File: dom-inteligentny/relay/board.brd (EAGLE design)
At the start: 92.7 x 87.6 mm, 77 parts, among them K1 OMRON-G3MB-202P-SSR, K10 OMRON-G3MB-202P-SSR, K11 OMRON-G3MB-202P-SSR, K12 OMRON-G3MB-202P-SSR, K13 OMRON-G3MB-202P-SSR, K14 OMRON-G3MB-202P-SSR, K15 OMRON-G3MB-202P-SSR, K16 OMRON-G3MB-202P-SSR, K17 691218410003, K18 691218410003, K19 691218410003, K2 OMRON-G3MB-202P-SSR, K20 691218410003, K21 691218410003, K22 691218410003, K3 OMRON-G3MB-202P-SSR, K4 OMRON-G3MB-202P-SSR, K5 OMRON-G3MB-202P-SSR, K6 OMRON-G3MB-202P-SSR, K7 OMRON-G3MB-202P-SSR, K8 OMRON-G3MB-202P-SSR, K9 OMRON-G3MB-202P-SSR, T1 BC847, T10 BC847, T11 BC847, T12 BC847, T13 BC847, T14 BC847, T15 BC847, T16 BC847, T2 BC847, T3 BC847, T4 BC847, T5 BC847, T6 BC847, T7 BC847, T8 BC847, T9 BC847, X1 GLX-S-88M

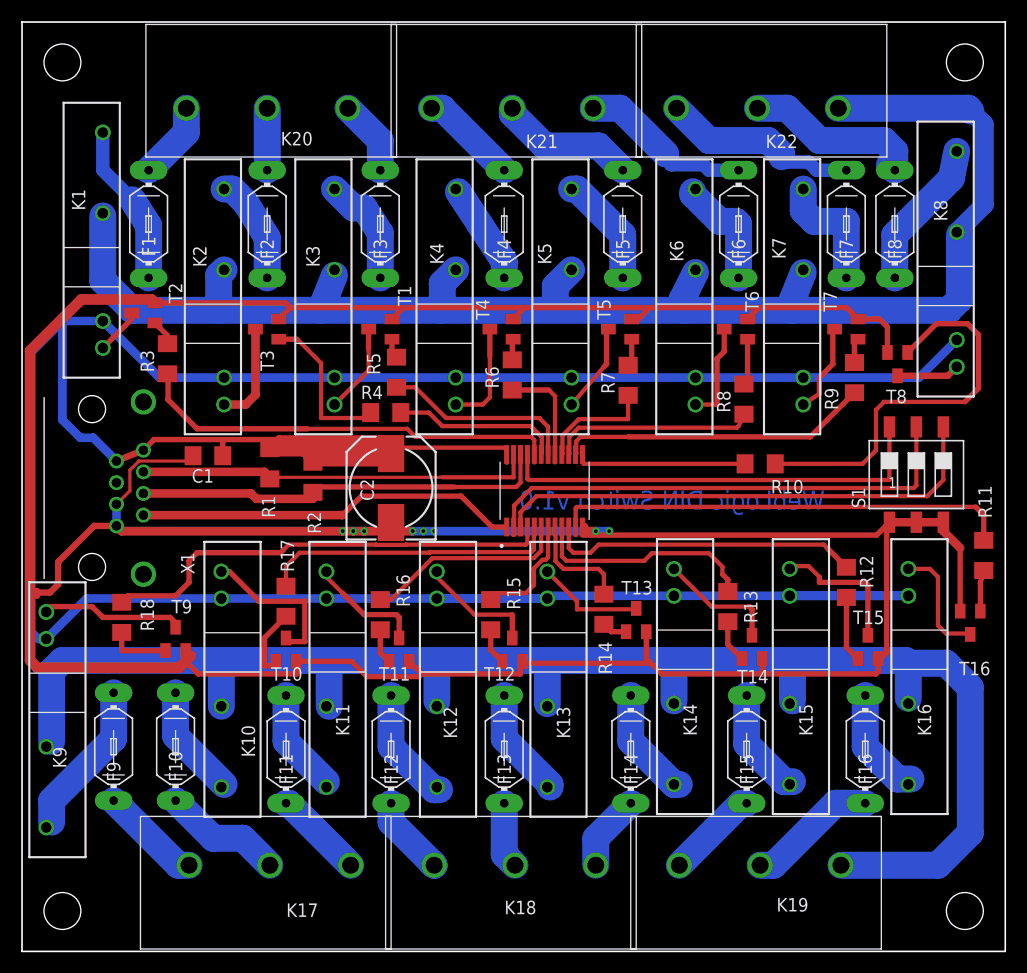
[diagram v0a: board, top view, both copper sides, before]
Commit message: new files
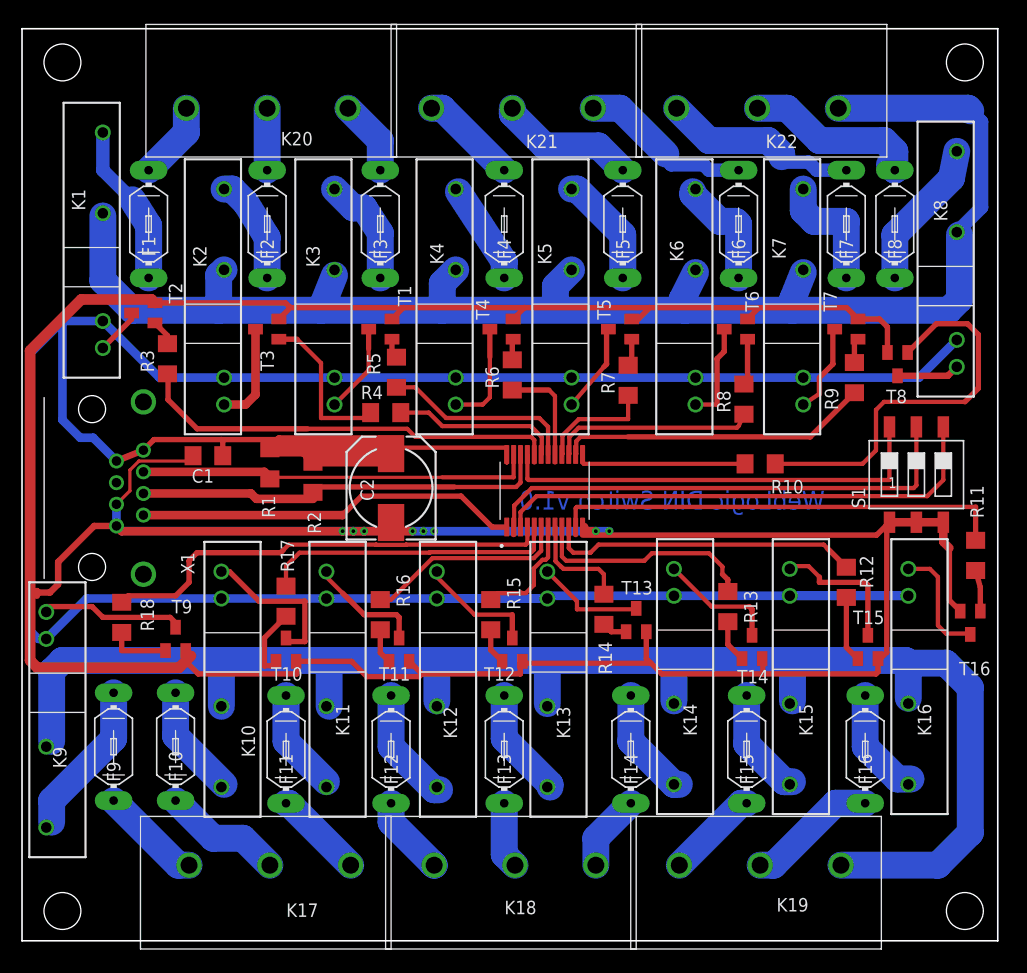
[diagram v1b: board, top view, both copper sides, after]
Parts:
- moved R11 0.76 mm to (89.9, 37.3)
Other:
- board size 92.7 x 87.6 mm -> 92 x 86 mm
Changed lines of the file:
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@@
 <setting verticaltext="up"/>
 </settings>
-<grid distance="10" unitdist="mil" unit="mil" style="lines" multiple="1" display="no" altdistance="5" altunitdist="mil" altunit="mil"/>
+<grid distance="1" unitdist="mm" unit="mm" style="lines" multiple="1" display="no" altdistance="1" altunitdist="mm" altunit="mm"/>
 <layers>
 <layer number="1" name="Top" color="4" fill="1" visible="yes" active="yes"/>
@@
 <board>
 <plain>
-<wire x1="0" y1="0" x2="0" y2="87.63" width="0.1524" layer="20"/>
-<wire x1="0" y1="87.63" x2="92.71" y2="87.63" width="0.1524" layer="20"/>
-<wire x1="92.71" y1="87.63" x2="92.71" y2="0" width="0.1524" layer="20"/>
-<wire x1="92.71" y1="0" x2="0" y2="0" width="0.1524" layer="20"/>
+<wire x1="0" y1="1" x2="0" y2="87" width="0.1524" layer="20"/>
+<wire x1="0" y1="87" x2="92" y2="87" width="0.1524" layer="20"/>
+<wire x1="92" y1="87" x2="92" y2="1" width="0.1524" layer="20"/>
+<wire x1="92" y1="1" x2="0" y2="1" width="0.1524" layer="20"/>
 <hole x="3.81" y="83.82" drill="3.4798"/>
 <hole x="88.9" y="83.82" drill="3.4798"/>
@@
 <attribute name="VALUE" x="68.326" y="43.434" size="1.27" layer="27"/>
 </element>
-<element name="R11" library="eagle-ltspice" library_urn="urn:adsk.eagle:library:217" package="R1206" package3d_urn="urn:adsk.eagle:package:13301/1" value="" x="90.678" y="37.338" smashed="yes" rot="R270">
-<attribute name="NAME" x="90.17" y="43.942" size="1.27" layer="25" rot="R270"/>
-<attribute name="SPICEMODEL" value="NONE" x="90.678" y="37.338" size="1.778" layer="27" rot="R270" display="off"/>
-<attribute name="SPICEPREFIX" value="R" x="90.678" y="37.338" size="1.778" layer="27" rot="R270" display="off"/>
-<attribute name="VALUE" x="88.138" y="38.608" size="1.27" layer="27" rot="R270"/>
+<element name="R11" library="eagle-ltspice" library_urn="urn:adsk.eagle:library:217" package="R1206" package3d_urn="urn:adsk.eagle:package:13301/1" value="" x="89.916" y="37.338" smashed="yes" rot="R270">
+<attribute name="NAME" x="89.408" y="43.942" size="1.27" layer="25" rot="R270"/>
+<attribute name="SPICEMODEL" value="NONE" x="89.916" y="37.338" size="1.778" layer="27" rot="R270" display="off"/>
+<attribute name="SPICEPREFIX" value="R" x="89.916" y="37.338" size="1.778" layer="27" rot="R270" display="off"/>
+<attribute name="VALUE" x="87.376" y="38.608" size="1.27" layer="27" rot="R270"/>
 </element>
 <element name="R12" library="eagle-ltspice" library_urn="urn:adsk.eagle:library:217" package="R1206" package3d_urn="urn:adsk.eagle:package:13301/1" value="" x="77.724" y="34.798" smashed="yes" rot="R270">
@@
 <contactref element="T13" pad="2"/>
 <contactref element="T12" pad="2"/>
-<wire x1="86.868" y1="39.624" x2="86.868" y2="40.4622" width="0.8128" layer="1"/>
-<wire x1="86.868" y1="39.624" x2="88.458" y2="38.034" width="0.8128" layer="1"/>
-<wire x1="88.458" y1="38.034" x2="88.458" y2="32.088" width="0.508" layer="1"/>
+<wire x1="86.868" y1="38.608" x2="86.868" y2="40.4622" width="0.8128" layer="1"/>
+<wire x1="86.868" y1="38.608" x2="87.442" y2="38.034" width="0.8128" layer="1"/>
+<wire x1="87.442" y1="38.034" x2="87.442" y2="33.104" width="0.508" layer="1"/>
+<wire x1="87.442" y1="33.104" x2="88.458" y2="32.088" width="0.508" layer="1"/>
 <wire x1="81.4578" y1="40.132" x2="81.788" y2="40.4622" width="0.508" layer="1"/>
 <wire x1="81.788" y1="40.4622" x2="80.5778" y2="39.252" width="0.508" layer="1"/>
@@
 <wire x1="73.66" y1="64.008" x2="72.644" y2="61.468" width="2.54" layer="16"/>
 <wire x1="72.644" y1="61.468" x2="72.644" y2="60.452" width="2.54" layer="16"/>
-<wire x1="88.138" y1="67.818" x2="90.7288" y2="70.4088" width="1.778" layer="16"/>
-<wire x1="90.7288" y1="70.4088" x2="90.7288" y2="77.978" width="1.778" layer="16"/>
-<wire x1="89.4588" y1="79.248" x2="90.7288" y2="77.978" width="1.778" layer="16"/>
+<wire x1="88.138" y1="67.818" x2="90.4748" y2="70.1548" width="1.27" layer="16"/>
+<wire x1="90.4748" y1="70.1548" x2="90.4748" y2="78.232" width="1.27" layer="16"/>
+<wire x1="89.4588" y1="79.248" x2="90.4748" y2="78.232" width="1.27" layer="16"/>
 <wire x1="51.816" y1="64.262" x2="50.292" y2="62.738" width="2.54" layer="16"/>
 <wire x1="50.292" y1="62.738" x2="50.292" y2="61.214" width="2.54" layer="16"/>
@@
 <contactref element="U$1" pad="11"/>
 <contactref element="R11" pad="1"/>
-<wire x1="89.916" y1="41.91" x2="90.678" y2="41.148" width="0.508" layer="1"/>
-<wire x1="90.678" y1="41.148" x2="90.678" y2="38.76" width="0.508" layer="1"/>
+<wire x1="89.916" y1="41.91" x2="89.916" y2="38.76" width="0.508" layer="1"/>
 <wire x1="52.201" y1="39.252" x2="52.201" y2="41.787" width="0.4064" layer="1"/>
 <wire x1="52.201" y1="41.787" x2="52.324" y2="41.91" width="0.4064" layer="1"/>
@@
 <contactref element="R11" pad="2"/>
 <contactref element="T16" pad="1"/>
-<wire x1="90.358" y1="32.088" x2="90.358" y2="34.762" width="0.508" layer="1"/>
-<wire x1="90.358" y1="34.762" x2="90.678" y2="35.916" width="0.508" layer="1"/>
+<wire x1="90.358" y1="32.088" x2="90.358" y2="34.3220375" width="0.508" layer="1"/>
+<wire x1="90.358" y1="34.3220375" x2="89.916" y2="35.916" width="0.508" layer="1"/>
 </signal>
 <signal name="N$83">
